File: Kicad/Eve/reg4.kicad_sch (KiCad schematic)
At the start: 11 parts, among them J8 Conn_01x03, J9 Conn_01x03

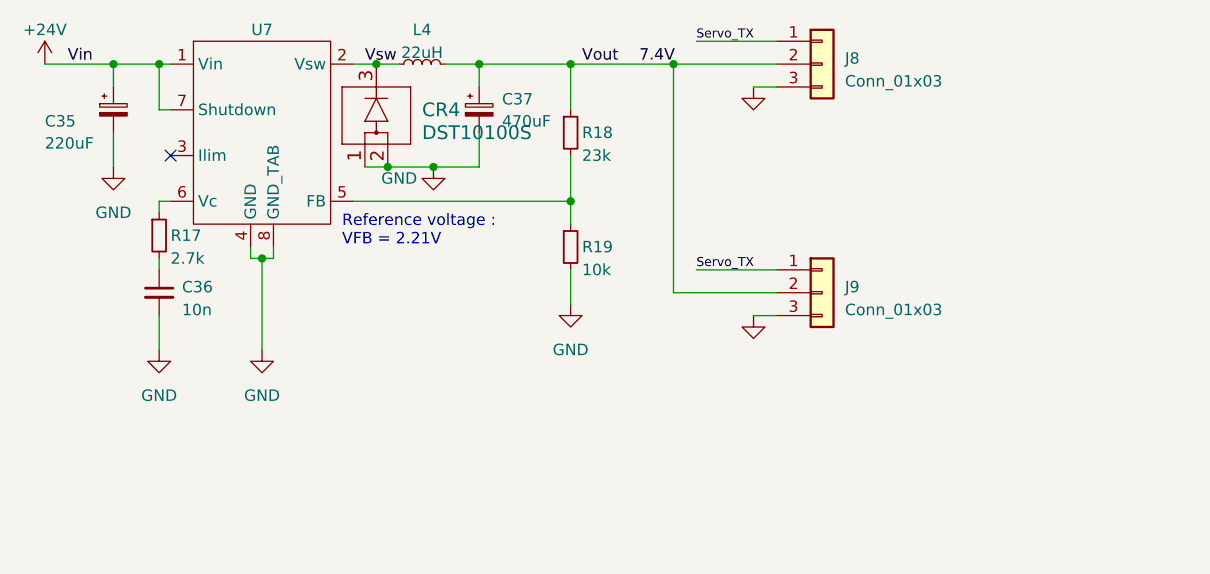
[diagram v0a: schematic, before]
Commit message: updtated Kicad ver 7.11.23
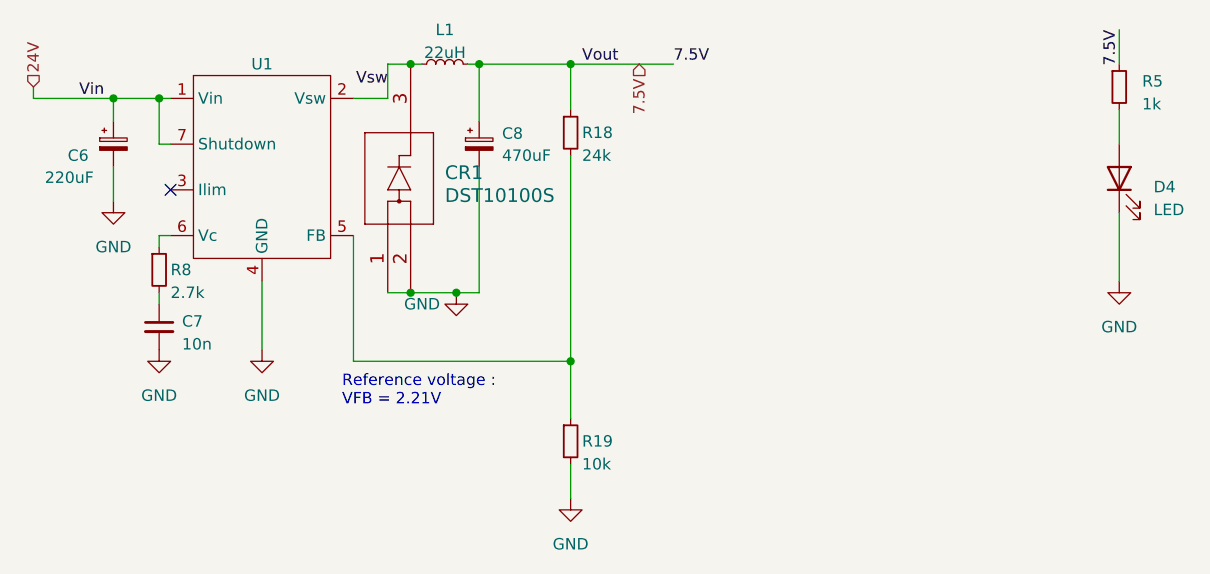
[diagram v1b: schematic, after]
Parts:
- removed C35: 220uF, Capacitor_SMD:CP_Elec_10x10.5, symbol Device:C_Polarized_Small
- removed C36: 10n, Capacitor_SMD:C_0603_1608Metric_Pad1.08x0.95mm_HandSolder, symbol Device:C_Small
- removed C37: 470uF, Capacitor_SMD:CP_Elec_10x10.5, symbol Device:C_Polarized_Small
- removed CR4: DST10100S, libs:DST10100S, symbol 2023-03-19_11-33-54:DST10100S
- removed J8, J9: Conn_01x03, symbol Connector_Generic:Conn_01x03
- removed L4: 22uH, Inductor_SMD:L_Wuerth_WE-PD-Typ-LS_Handsoldering, symbol Device:L_Small
- removed R17: 2.7k, Resistor_SMD:R_0603_1608Metric_Pad0.98x0.95mm_HandSolder, symbol Device:R_Small
- removed U7: ~, libs:LT1076CR-PBF, symbol custom:LT1076
- added C6: 220uF, Capacitor_SMD:CP_Elec_10x10.5, symbol Device:C_Polarized_Small
- added C7: 10n, Capacitor_SMD:C_0603_1608Metric_Pad1.08x0.95mm_HandSolder, symbol Device:C_Small
- added C8: 470uF, Capacitor_SMD:CP_Elec_10x10.5, symbol Device:C_Polarized_Small
- added CR1: DST10100S, TO277B_LTF, symbol 2023-03-19_11-33-54:DST10100S
- added D4: LED, LED_SMD:LED_0603_1608Metric_Pad1.05x0.95mm_HandSolder, symbol Device:LED
- added L1: 22uH, Inductor_SMD:L_Wuerth_WE-PD-Typ-LS_Handsoldering, symbol Device:L_Small
- added R5: 1k, Resistor_SMD:R_0603_1608Metric_Pad0.98x0.95mm_HandSolder, symbol Device:R_Small
- added R8: 2.7k, Resistor_SMD:R_0603_1608Metric_Pad0.98x0.95mm_HandSolder, symbol Device:R_Small
- added U1: ~, symbol custom:LT1076
- R18: value 23k -> 24k
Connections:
- net GND: now also C6.2, C7.2, C8.2, CR1.1, CR1.2, D4.1 (K), U1.4 (GND)
- net Vsw: now also CR1.3, L1.1, U1.2 (Vsw)
- net at R18.2, R19.1: now also U1.5 (FB)
- net 7.4V renamed 7.5V
- net 7.5V: now also C8.1, L1.2, R5.1
- new net: R8.1, U1.6 (Vc)
- new net: C7.1, R8.2
- new net: D4.2 (A), R5.2
- new net 24V: C6.1, U1.1 (Vin), U1.7 (Shutdown)
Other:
- moved on the sheet: R19
